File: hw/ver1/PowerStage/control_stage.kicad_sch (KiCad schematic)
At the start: 3 parts, among them J10 SWD Debug, P1 USB_C_Plug_USB2.0, U10 RP2040

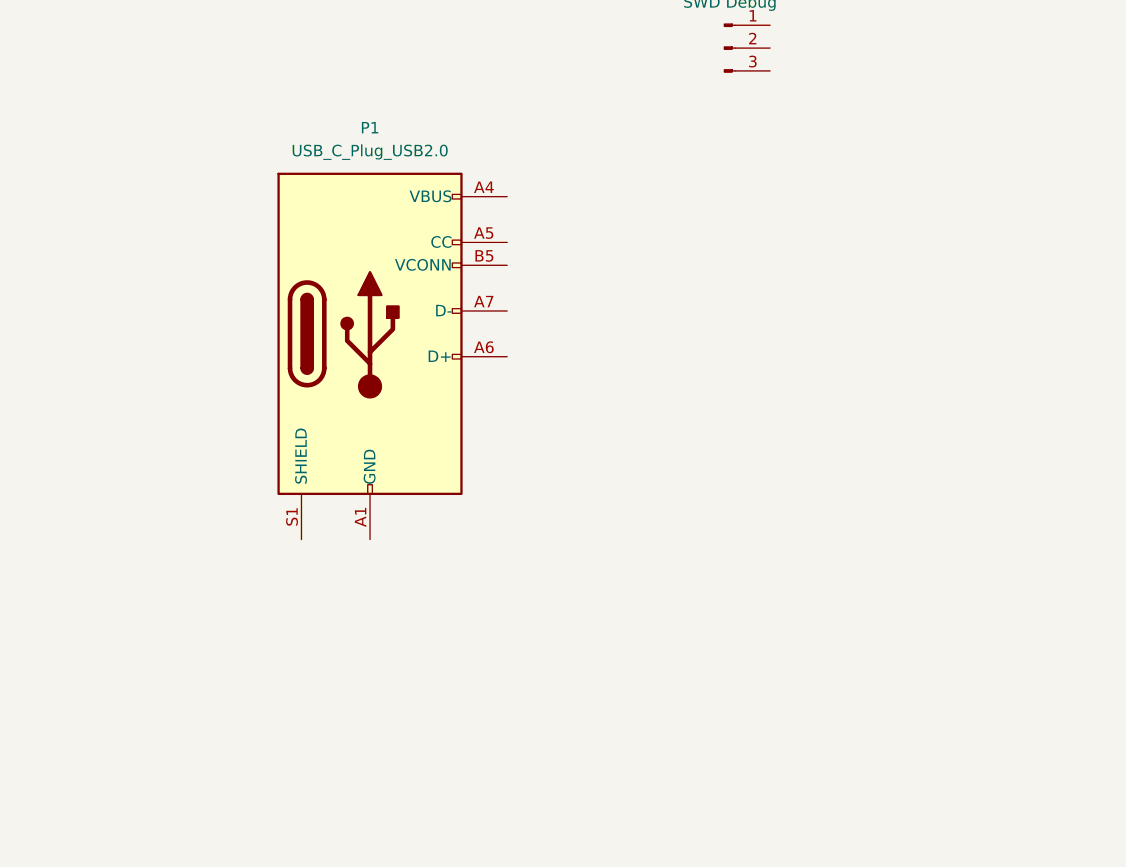
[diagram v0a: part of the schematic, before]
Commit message: Sync morning work to laptop
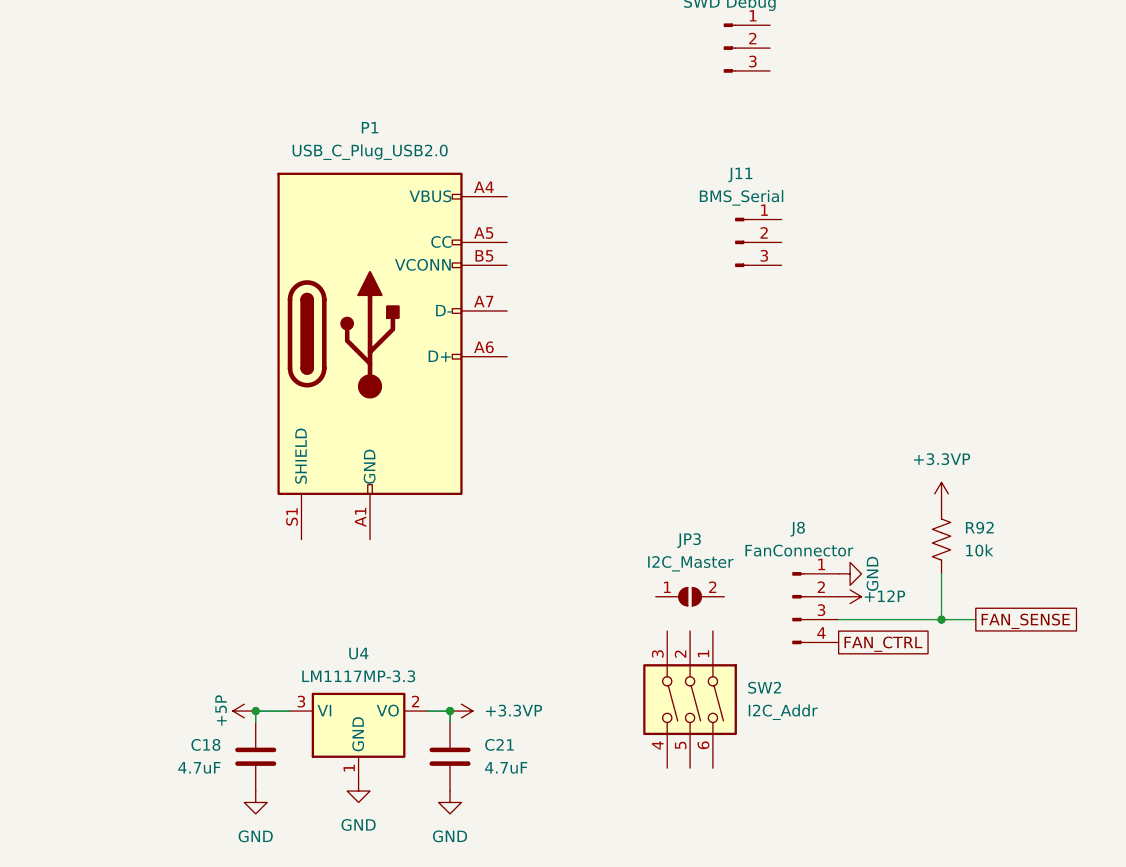
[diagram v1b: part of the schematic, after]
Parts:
- added C18, C21: 4.7uF, Capacitor_SMD:C_0603_1608Metric, symbol Device:C
- added J11: BMS_Serial, Connector_PinHeader_2.54mm:PinHeader_1x03_P2.54mm_Vertical, symbol Connector:Conn_01x03_Pin
- added J8: FanConnector, Connector_Molex:Molex_KK-254_AE-6410-04A_1x04_P2.54mm_Vertical, symbol Connector:Conn_01x04_Pin
- added JP3: I2C_Master, symbol Jumper:SolderJumper_2_Open
- added R92: 10k, Resistor_SMD:R_0603_1608Metric, symbol Device:R_US
- added SW2: I2C_Addr, Button_Switch_SMD:SW_DIP_SPSTx03_Slide_6.7x9.18mm_W6.73mm_P2.54mm_LowProfile_JPin, symbol Switch:SW_DIP_x03
- added U4: LM1117MP-3.3, Package_TO_SOT_SMD:SOT-223-3_TabPin2, symbol Regulator_Linear:LM1117MP-3.3
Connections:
- new net +12P: J8.2 (Pin_2)
- new net +3.3VP: C21.1, R92.2, U4.2 (VO)
- new net +5P: C18.1, U4.3 (VI)
- new net FAN_CTRL: J8.4 (Pin_4)
- new net FAN_SENSE: J8.3 (Pin_3), R92.1
- new net GND: C18.2, C21.2, J8.1 (Pin_1), U4.1 (GND)
